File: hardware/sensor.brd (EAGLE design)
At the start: 35.8 x 35.8 mm, 32 parts, among them J1 MICRO_USB_B_HIROSE_ZX62-B-5PA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, J2 DM3AT-SF-PEJM5, SW1 TVAF06-A020B-R, X1 FA-238

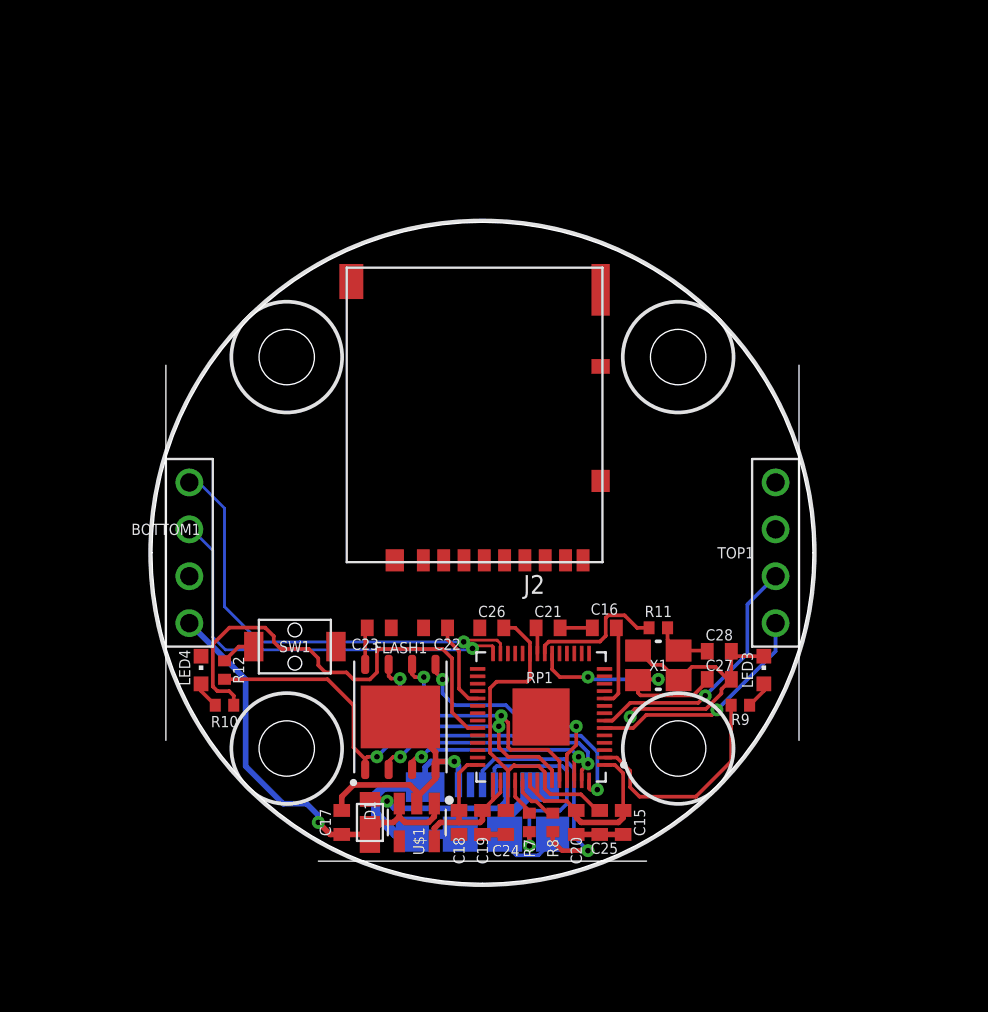
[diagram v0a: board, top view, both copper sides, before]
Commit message: WIP
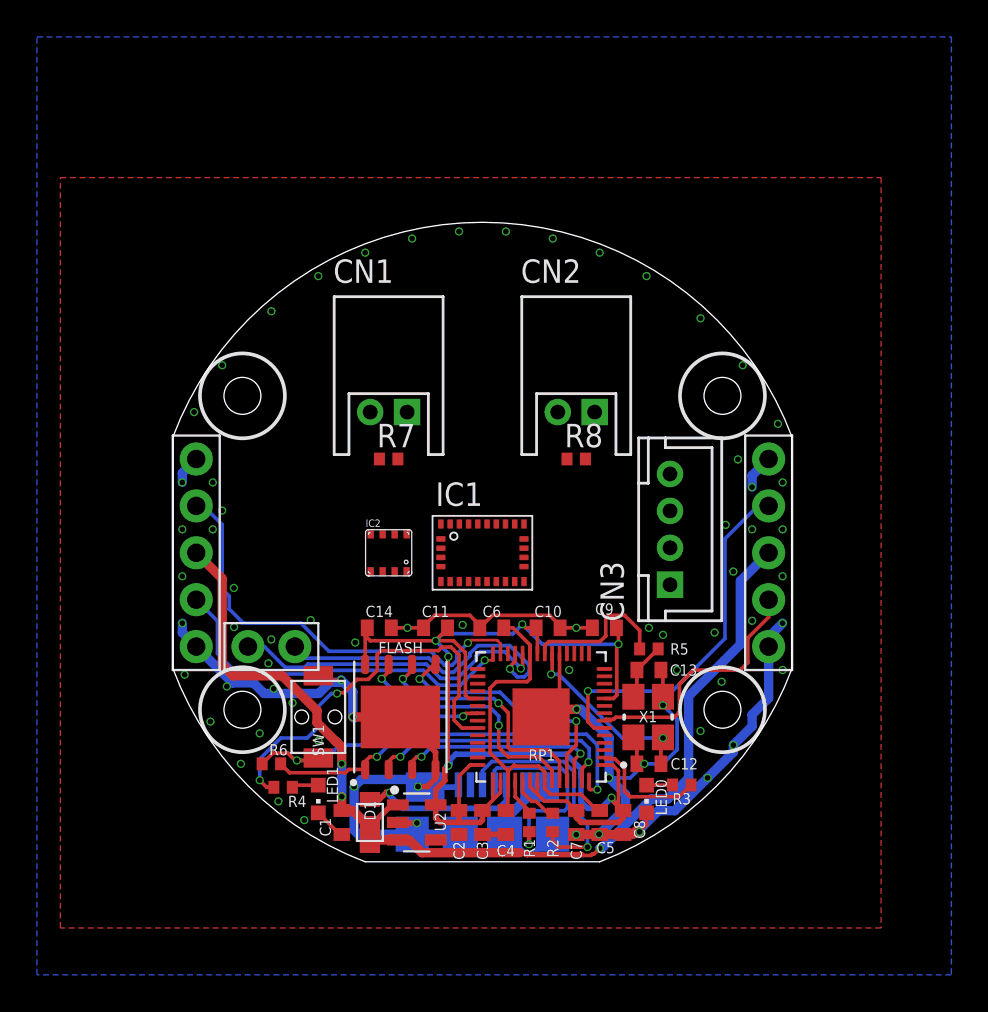
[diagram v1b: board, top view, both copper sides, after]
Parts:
- removed BOTTOM1, TOP1: P4_2.54, pins:P4_2.54
- removed C27, C28: (no value), rcl:C0402
- removed J2: DM3AT-SF-PEJM5, connector:DM3AT-SF-PEJM5
- removed LED3, LED4: (no value), led:CHIPLED_0603
- removed R10, R9: (no value), rcl:R0402
- removed R11, R12: 1k, rcl:R0402
- added BOTTOM, TOP: P5_2.54, pins:P5_2.54
- added C12, C13: (no value), rcl:C0402
- added CN1, CN2: (no value), jst-ph:S2B-PH-K-S
- added CN3: (no value), jst-ph:B4B-PH-K-S
- added IC1: BN055, BNO055:LGA-28_3.80X5.20/0.5
- added IC2: BME280, bosch-bme280:BME280
- added LED0, LED1: (no value), led:CHIPLED_0603
- added R1, R2, R3, R4: (no value), rcl:R0402
- added R5, R6: 1k, rcl:R0402
- added U$2: P2_2_2.54, pins:P2_2.54
- R7, R8: value (none) -> 22k
- moved R7 21.1 mm to (-5.08, 5.08), turned to 0 degrees
- moved R8 19.7 mm to (5.08, 5.08), turned to 0 degrees
- moved SW1 4.02 mm to (-8.89, -8.89), turned to 0 degrees
- moved X1 2.86 mm to (8.98, -8.90), turned to 270 degrees
- turned C1 to 270 degrees
- turned U2 to 0 degrees
- renumbered C15 to C8, C16 to C9, C17 to C1, C18 to C2, C19 to C3, C20 to C7, C21 to C10, C22 to C11, C23 to C14, C24 to C4, C25 to C5, C26 to C6, FLASH1 to FLASH, U$1 to U2
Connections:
- net I2C_SCL renamed I2C0_SCL
- net SPI0_RX renamed SPI0_MISO
- net SPI0_TX renamed SPI0_MOSI
- net SPI1_RX renamed SPI1_MISO
- net SPI1_TX renamed SPI1_MOSI
- removed net ADC0: RP1.38
- removed net ADC1: RP1.39
- removed net N$10: LED4.A, R10.1
- removed net N$12: R12.1, SW1.P$2
- removed net PWM3_B: RP1.35
- new net GND_IO: IC1.25
- new net N$8: LED0.A, R3.1
- new net SW: R6.1, RP1.35, SW1.P$2
- new net T0: CN2.2, R8.2, RP1.38
- new net T1: CN1.2, R7.2, RP1.39
- new net VDDIO: IC1.28, IC2.6
- net GND: now also BOTTOM.1, BOTTOM.5, C12.2, C13.2, CN3.2, IC1.2, IC2.1, IC2.7, LED0.C, LED1.C, R7.1, R8.1, TOP.1, TOP.5; no longer BOTTOM1.2, C27.2, C28.2, LED3.C, LED4.C, TOP1.2
- net I2C1_SCL: now also CN3.4
- net I2C1_SDA: now also CN3.3
- net LED0: now also R3.2; no longer R9.2
- net LED1: now also R4.2; no longer R10.2
- net N$11: now also C13.1, R5.1; no longer C28.1, R11.1
- net N$9: now also LED1.A, R4.1; no longer LED3.A, R9.1
- net QSPI_SS: now also R6.2; no longer R12.2
- net RX0: now also TOP.4; no longer BOTTOM1.3
- net RX1: now also BOTTOM.4; no longer TOP1.3
- net SWCLK: now also U$2.P$1
- net SWD: now also U$2.P$2
- net TX0: now also TOP.2; no longer BOTTOM1.4
- net TX1: now also BOTTOM.2; no longer TOP1.4
- net USB_DM: now also R1.2; no longer R7.2
- net USB_DM_1: now also R1.1; no longer R7.1
- net USB_DP: now also R2.2; no longer R8.2
- net USB_DP_1: now also R2.1; no longer R8.1
- net V+: now also BOTTOM.3, TOP.3; no longer BOTTOM1.1, TOP1.1
- net VDD: now also CN1.1, CN2.1, CN3.1, IC1.3, IC2.8
- net XIN1: now also C12.1; no longer C27.1
- net XOUT1: now also R5.2; no longer R11.2
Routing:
- net GND: track 57.6 -> 112.9 mm, vias 2 -> 71
- net VDD: track 34.5 -> 73.0 mm, vias 0 -> 6
- net V+: track 23.1 -> 57.0 mm, vias 1 -> 3
- net SWCLK: track 0.00 -> 17.6 mm, vias 0 -> 1
- net SWD: track 0.00 -> 17.1 mm, vias 0 -> 1
- net SW: track 0.00 -> 14.3 mm, vias 0 -> 2
- net TX1: track 12.5 -> 19.8 mm
- net QSPI_SS: track 27.7 -> 22.0 mm
- net LED0: track 12.1 -> 6.55 mm
- net LED1: track 25.3 -> 21.8 mm, vias 0 -> 2
- net XIN1: track 12.9 -> 10.2 mm
- net RX0: track 22.4 -> 20.1 mm
- net N$12: track 1.90 -> 0.00 mm, vias 0 -> 1
- net N$10: track 1.47 -> 0.00 mm
- net N$8: track 0.00 -> 1.41 mm
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- added copper zone on layer 1, net GND
- added copper zone on layer 16, net GND
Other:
- board size 35.8 x 35.8 mm -> 33.5 x 34.6 mm
- board text added: "2022 WASA Rocket"
- board text added: "TERES Module"
